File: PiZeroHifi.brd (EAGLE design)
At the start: 100 x 80 mm, 45 parts, among them CON1 RPI-ZEROPI-ZERO-THRUHOLE, CON3 Audio Out, J1 GROVEGROVE-HORIZONTAL, J2 GROVEGROVE-HORIZONTAL, J3 GROVEGROVE-HORIZONTAL, U1 TXS0102, U2 LSM6DS33, U3 TC1014-3.3V, U4 PCM5101A, U5 PAM8403, U6 TXB0104PWR

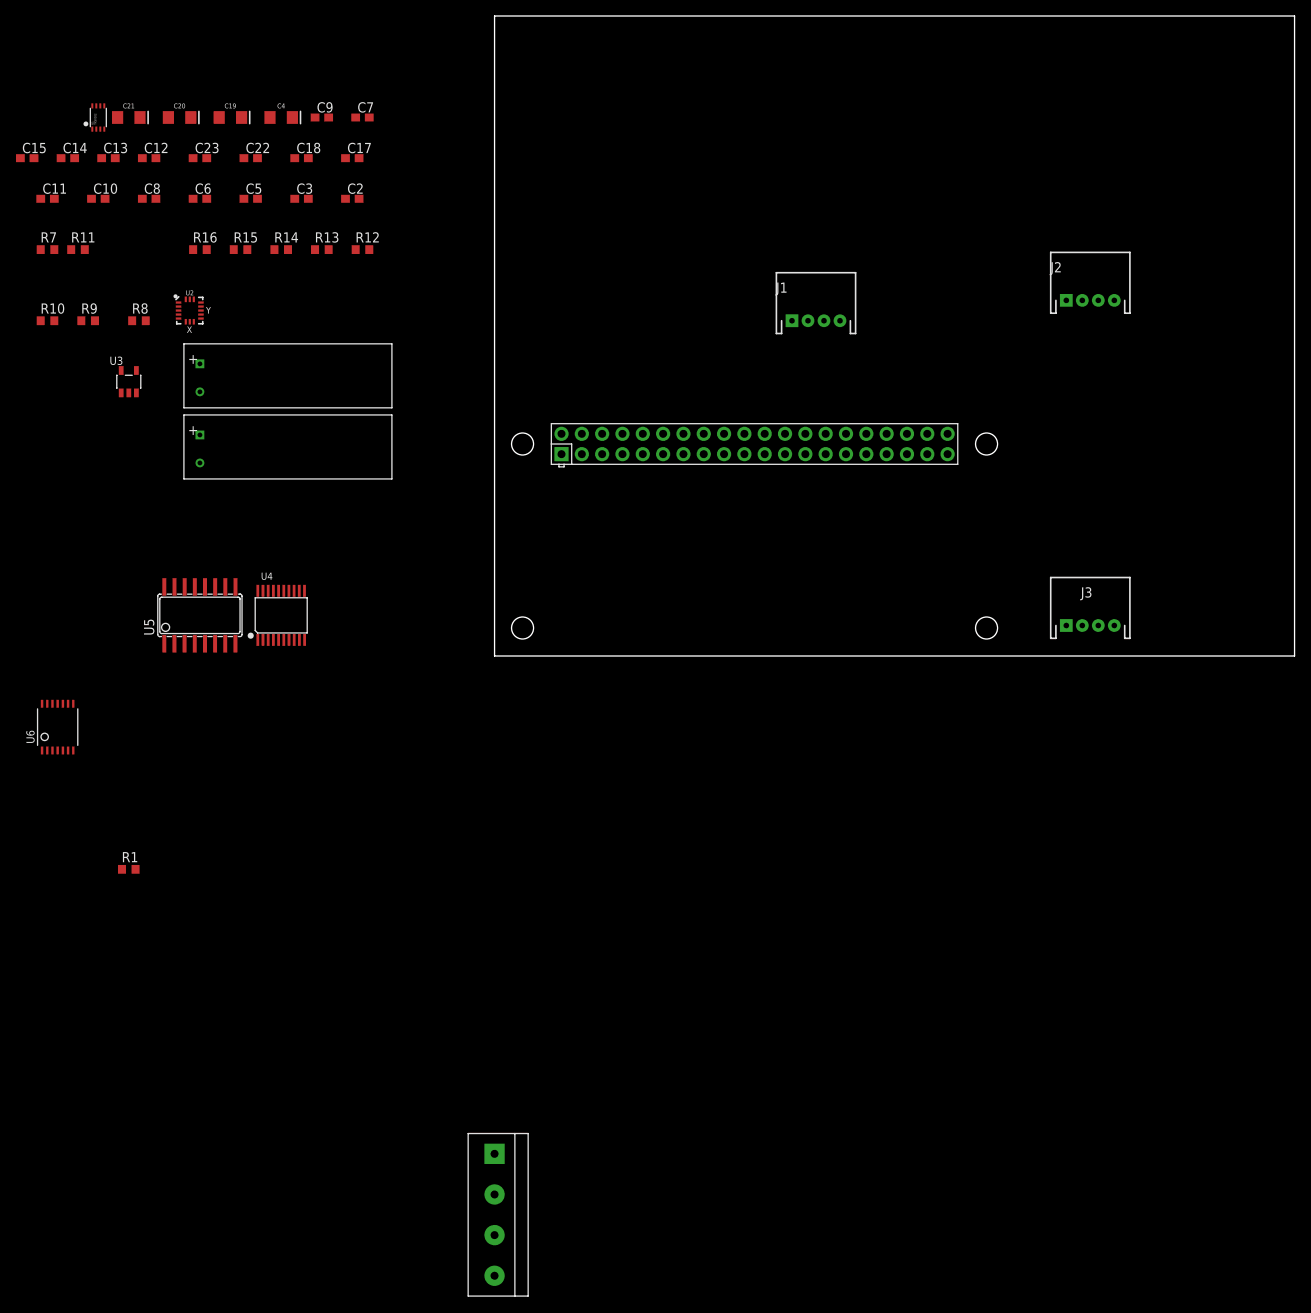
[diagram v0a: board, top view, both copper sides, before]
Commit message: Added Hifi Board
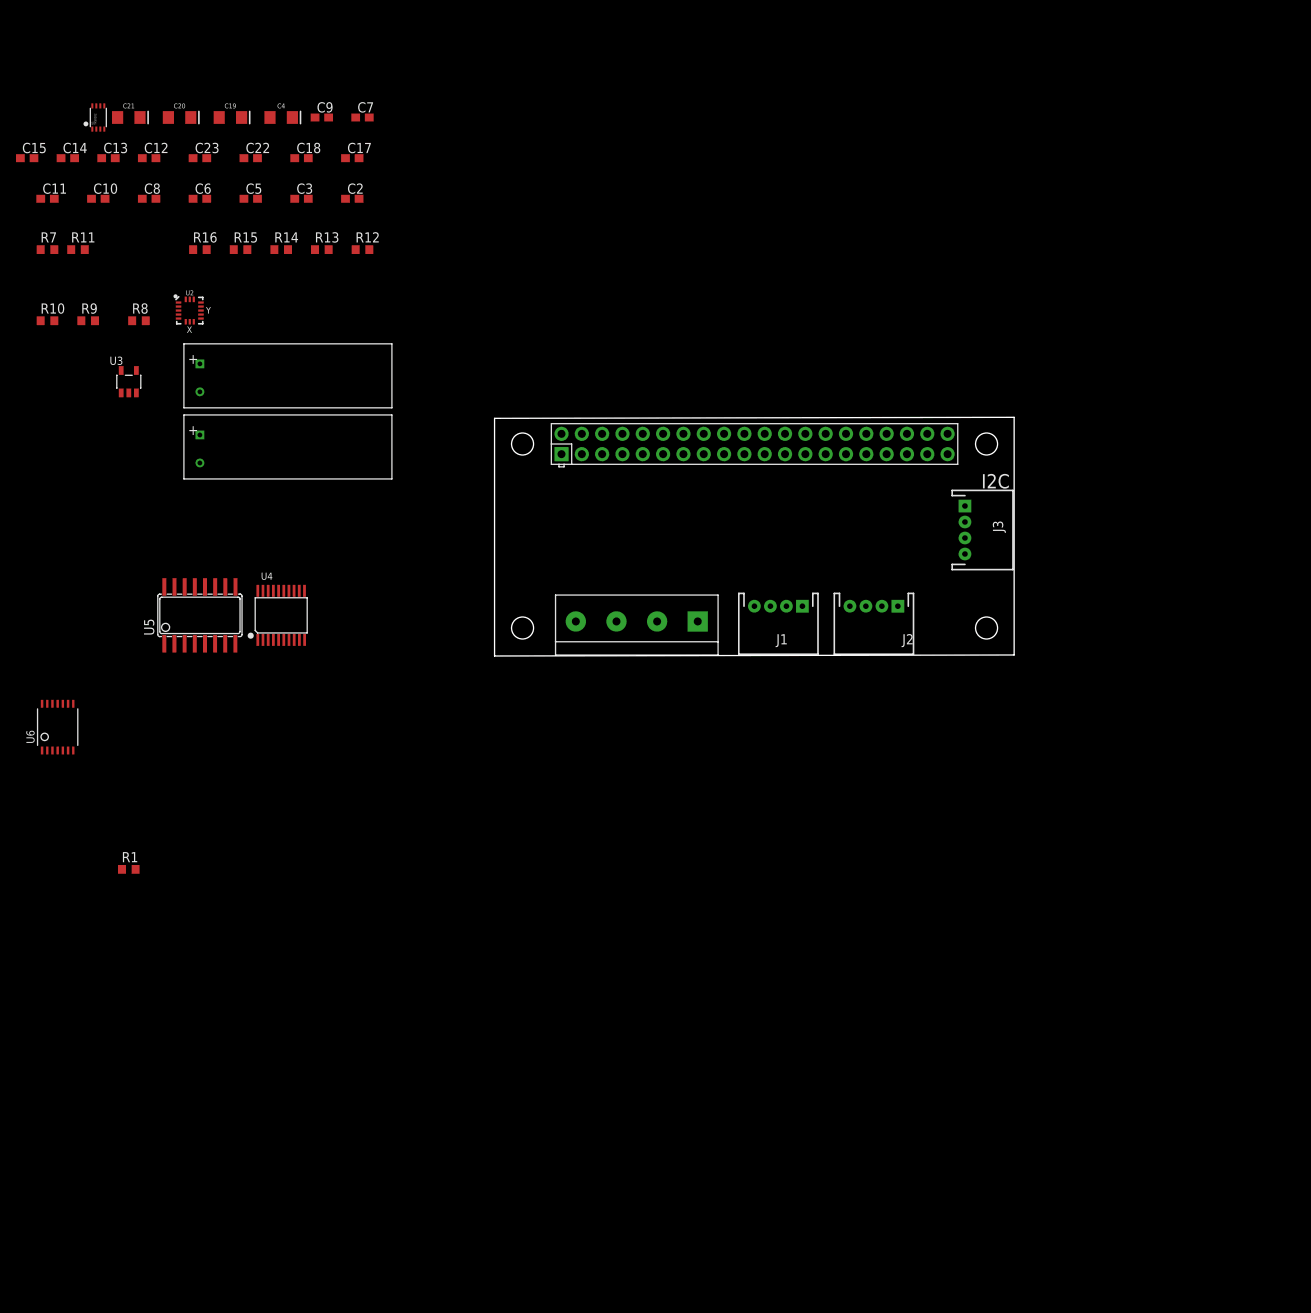
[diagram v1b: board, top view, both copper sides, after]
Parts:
- moved CON3 74.5 mm to (20.3, 4.32), turned to 270 degrees
- moved J2 46.8 mm to (47.4, 6.22), turned to 180 degrees
- moved J1 36.0 mm to (35.5, 6.22), turned to 180 degrees
- moved J3 19.7 mm to (58.8, 15.7), turned to 270 degrees
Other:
- board size 100 x 80 mm -> 64.9 x 29.8 mm
- board text added: "I2C"

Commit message: Revert "Added Hifi Board"
This reverts commit 465897fff771744b6bd4fb0467af0f24cf217bbb.
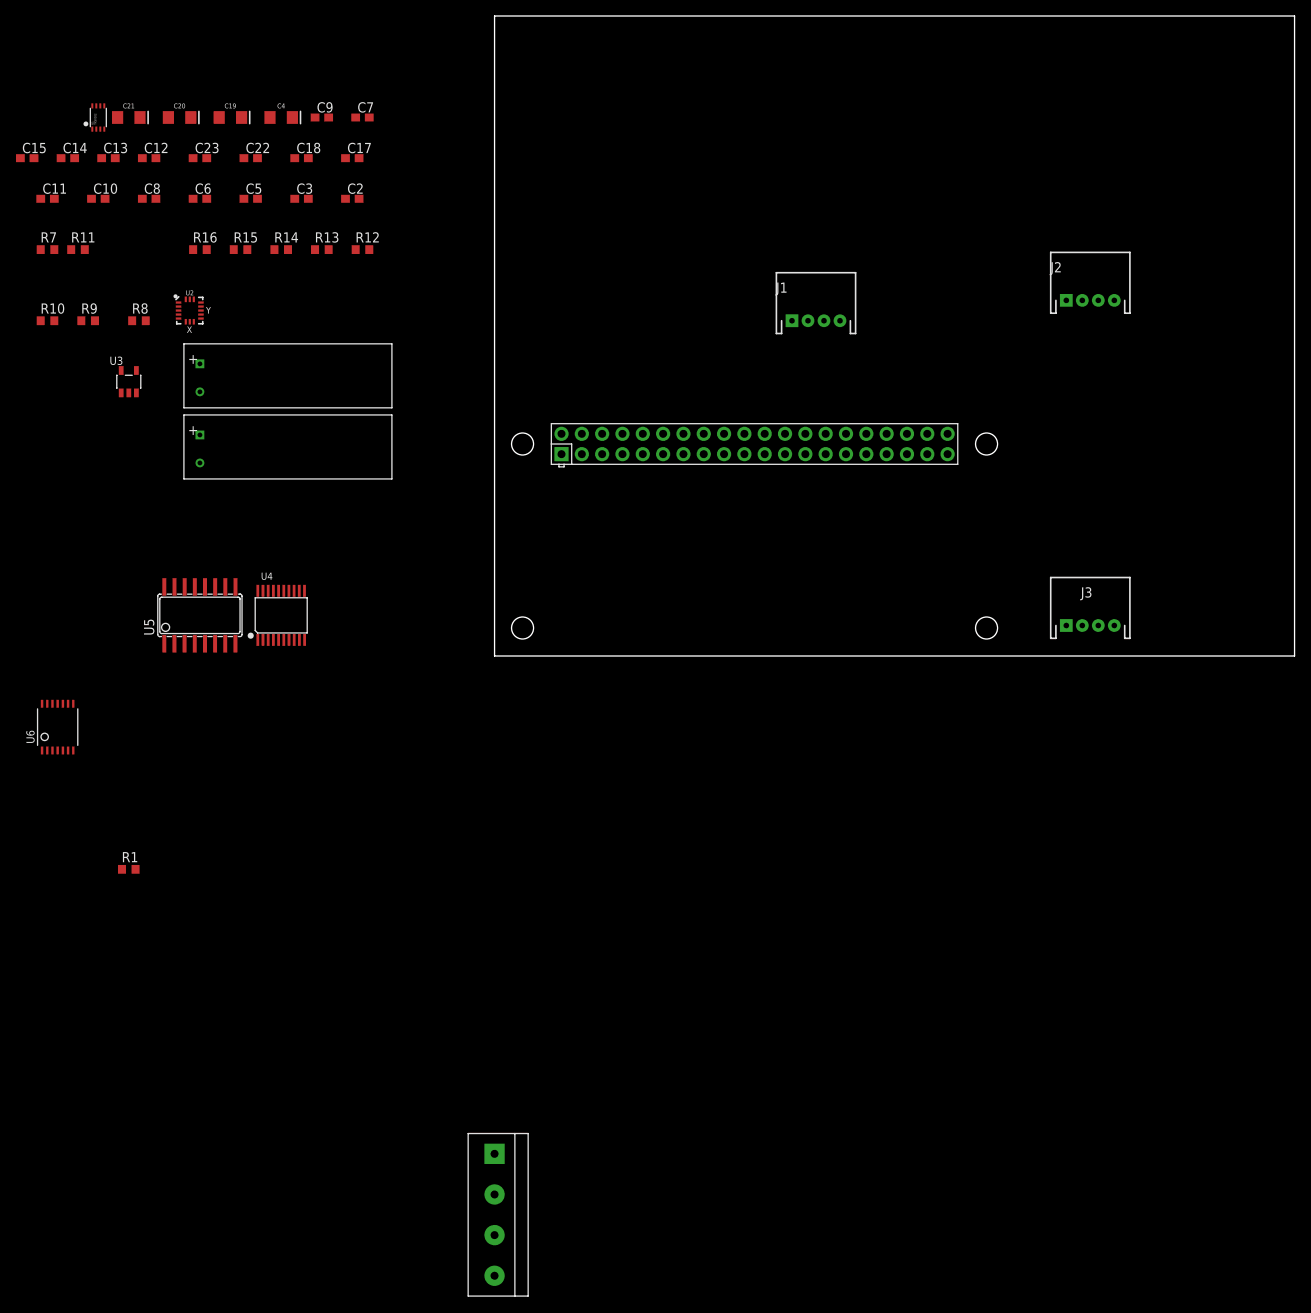
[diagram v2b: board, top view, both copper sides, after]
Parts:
- moved CON3 74.5 mm to (0.00, -67.3), turned to 0 degrees
- moved J2 46.8 mm to (74.5, 44.5), turned to 0 degrees
- moved J1 36.0 mm to (40.2, 41.9), turned to 0 degrees
- moved J3 19.7 mm to (74.5, 3.81), turned to 0 degrees
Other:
- board size 64.9 x 29.8 mm -> 100 x 80 mm
- board text removed: "I2C"
